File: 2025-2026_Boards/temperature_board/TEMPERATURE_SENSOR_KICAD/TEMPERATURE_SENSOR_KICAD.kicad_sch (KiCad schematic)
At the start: 53 parts, among them J1 LCD Connector Pinout, U1 STM32G431CBT6, U2 TMP235A4DBZR, U3 AMS1117-3.3, U5 TPS62932DRLR, U6 TPS62932DRLR, U8 AMS1117

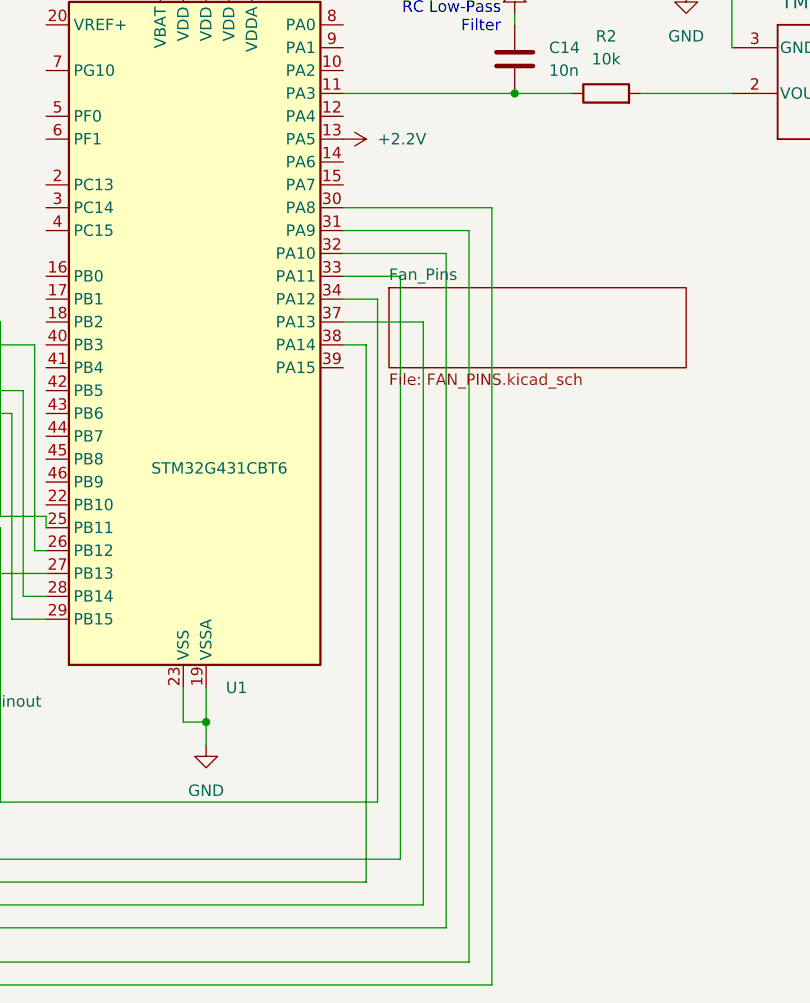
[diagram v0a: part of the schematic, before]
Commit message: minor updates
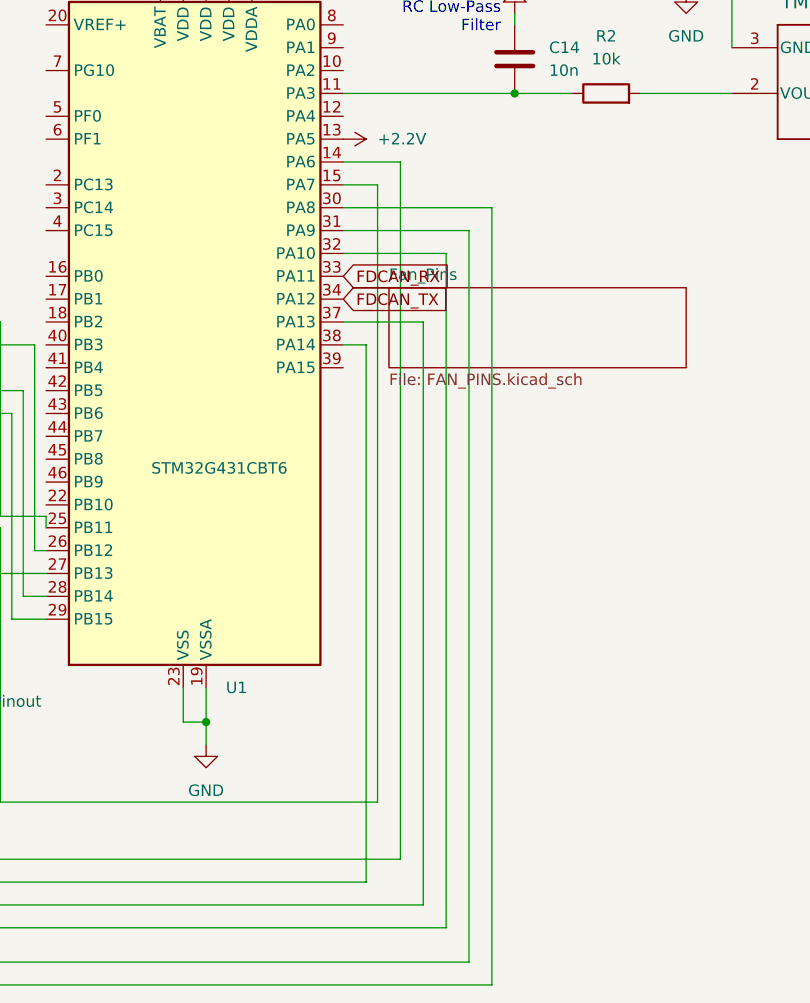
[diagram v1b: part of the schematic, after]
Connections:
- net at U1.14 (PA6): now also J1.9 (Pin_9)
- net at U1.15 (PA7): now also J1.10 (Pin_10)
- net FDCAN_RX: now reaches U1.33 (PA11)
- net FDCAN_RX: no longer J1.9 (Pin_9)
- net FDCAN_TX: now reaches U1.34 (PA12)
- net FDCAN_TX: no longer J1.10 (Pin_10)
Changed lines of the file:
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@@
-	(wire
-		(pts
-			(xy 128.27 118.11) (xy 124.46 118.11)
-		)
-		(stroke
-			(width 0)
-			(type default)
-		)
-	)
 	(wire
 		(pts
@@
 	(wire
 		(pts
-			(xy 130.81 115.57) (xy 124.46 115.57)
-		)
-		(stroke
-			(width 0)
-			(type default)
-		)
-	)
-	(wire
-		(pts
 			(xy 90.17 123.19) (xy 90.17 146.05)
 		)
@@
 	(wire
 		(pts
+			(xy 128.27 105.41) (xy 124.46 105.41)
+		)
+		(stroke
+			(width 0)
+			(type default)
+		)
+	)
+	(wire
+		(pts
 			(xy 86.36 120.65) (xy 86.36 142.24)
 		)
@@
 	(wire
 		(pts
-			(xy 130.81 180.34) (xy 130.81 115.57)
+			(xy 130.81 102.87) (xy 130.81 180.34)
 		)
 		(stroke
@@
 	(wire
 		(pts
-			(xy 128.27 173.99) (xy 128.27 118.11)
+			(xy 128.27 105.41) (xy 128.27 173.99)
 		)
 		(stroke
@@
 		(pts
 			(xy 106.68 74.93) (xy 106.68 82.55)
+		)
+		(stroke
+			(width 0)
+			(type default)
+		)
+	)
+	(wire
+		(pts
+			(xy 130.81 102.87) (xy 124.46 102.87)
 		)
 		(stroke
@@
 		)
 	)
+	(global_label "FDCAN_TX"
+		(shape input)
+		(at 124.46 118.11 0)
+		(fields_autoplaced yes)
+		(effects
+			(font
+				(size 1.27 1.27)
+			)
+			(justify left)
+		)
+		(property "Intersheetrefs" "${INTERSHEET_REFS}"
+			(at 136.6376 118.11 0)
+			(effects
+				(font
+					(size 1.27 1.27)
+				)
+				(justify left)
+				(hide yes)
+			)
+		)
+	)
+	(global_label "FDCAN_RX"
+		(shape input)
+		(at 124.46 115.57 0)
+		(fields_autoplaced yes)
+		(effects
+			(font
+				(size 1.27 1.27)
+			)
+			(justify left)
+		)
+		(property "Intersheetrefs" "${INTERSHEET_REFS}"
+			(at 136.94 115.57 0)
+			(effects
+				(font
+					(size 1.27 1.27)
+				)
+				(justify left)
+				(hide yes)
+			)
+		)
+	)

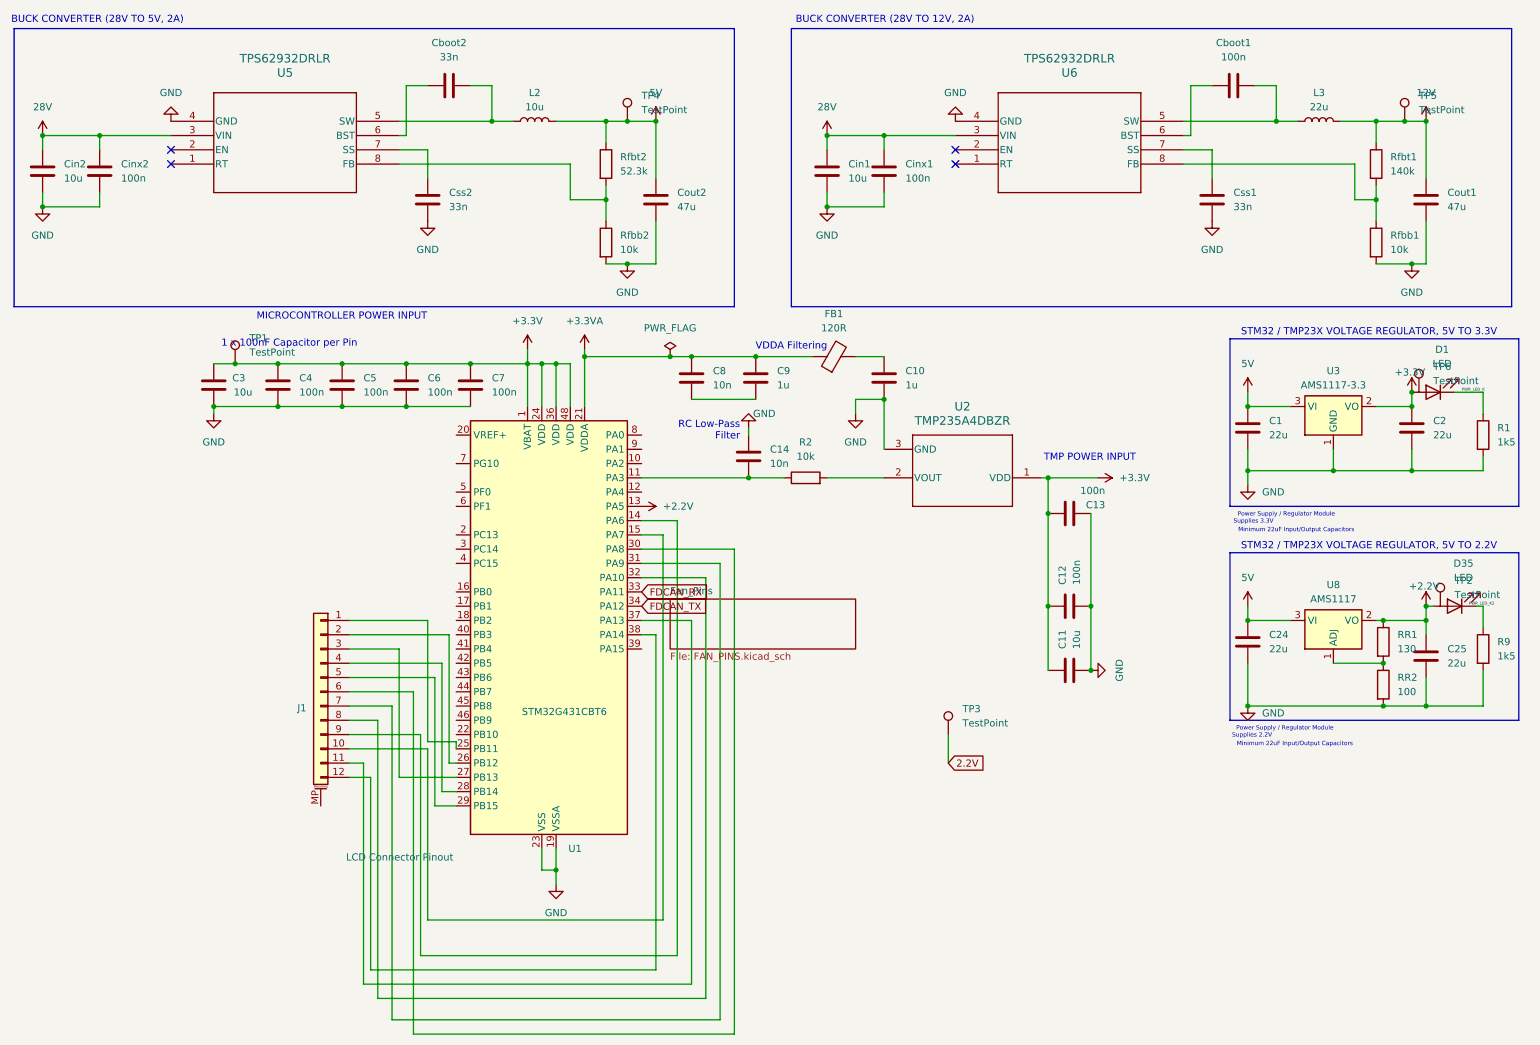
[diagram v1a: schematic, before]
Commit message: finishing the board. debuggign,ectc
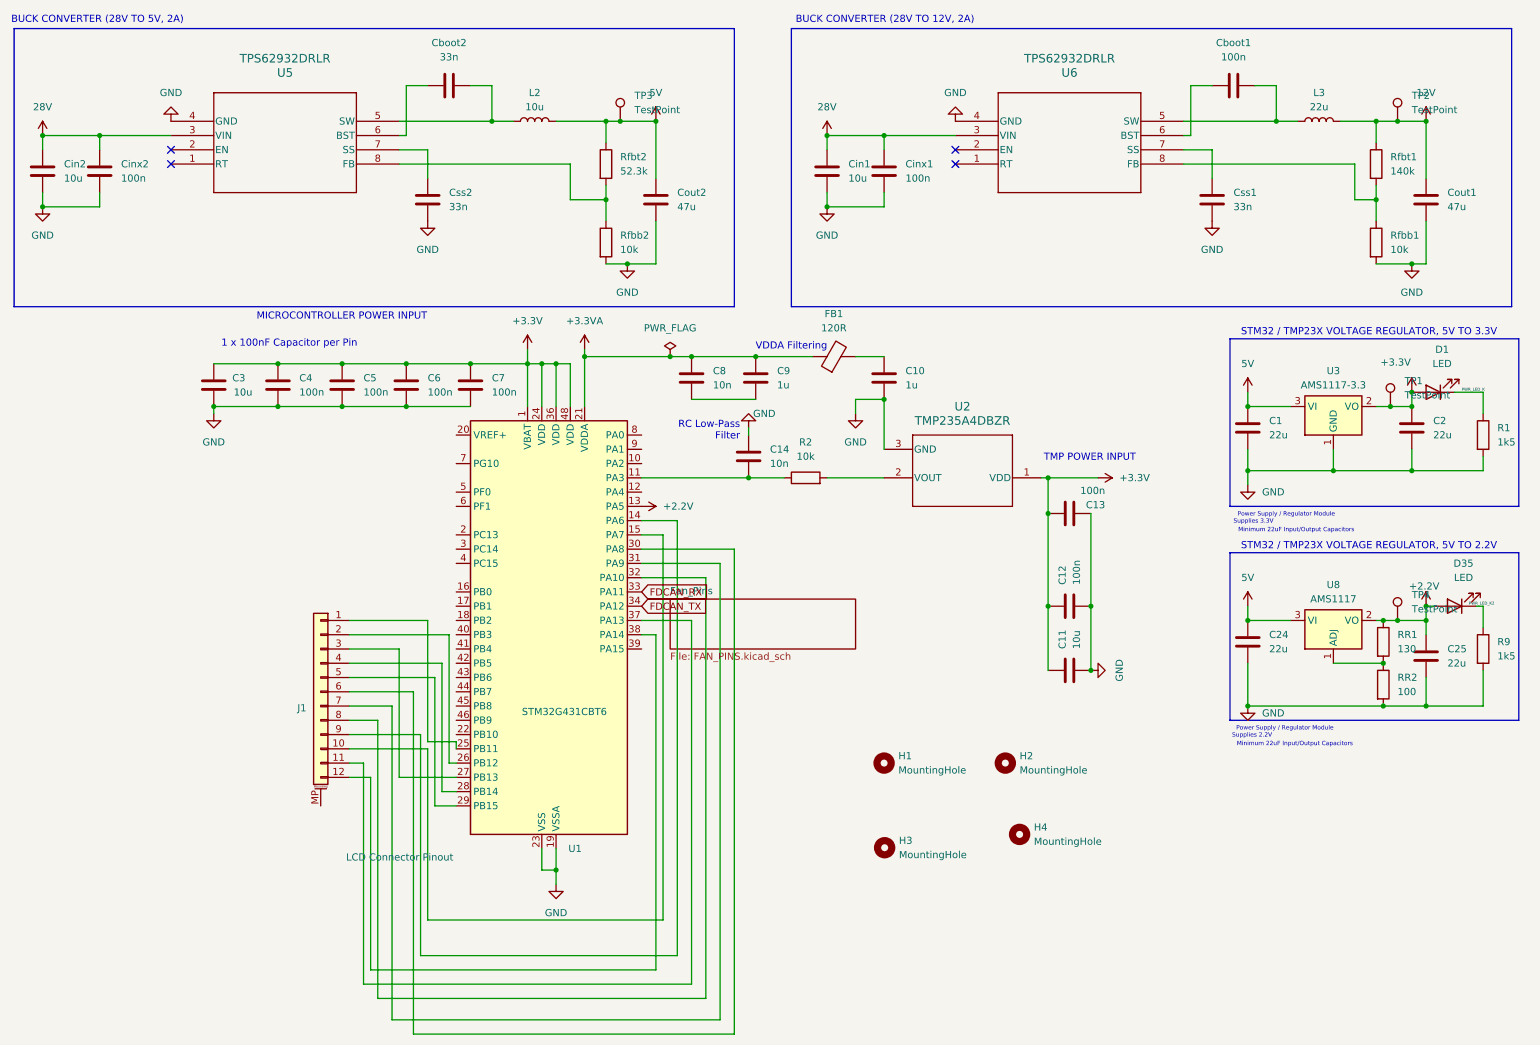
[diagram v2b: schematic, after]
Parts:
- removed TP5, TP6: TestPoint, symbol Connector:TestPoint
- added H1, H2, H3, H4: MountingHole, MountingHole:MountingHole_4.3mm_M4, symbol Mechanical:MountingHole
- TP1, TP2, TP3, TP4: footprint (none) -> Connector_Pin:Pin_D1.3mm_L10.0mm_W3.5mm_Flat
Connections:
- net 2.2V is gone; now on net 5V: TP3.1
- net +2.2V: now also TP4.1
- net 12V: now also TP2.1
- net 5V: no longer TP4.1
